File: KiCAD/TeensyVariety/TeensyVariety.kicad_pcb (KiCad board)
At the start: 2 copper layers, 49.5 x 40.5 mm, 36 parts, among them J1 CH1, J2 TRIG INP, J3 LASER, J4 CH2, J5 CH3, J6 CH4 / Decimated Trig, J7 DEBUG, J8 PHOTOTRANSISTOR, Q2 Q_NPN_BCE, U1 Teensy4.0

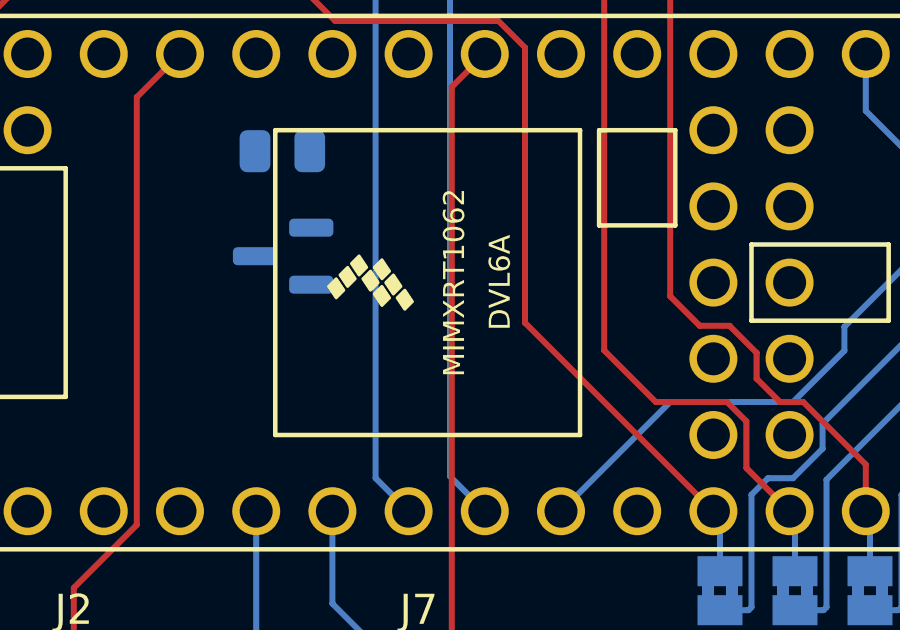
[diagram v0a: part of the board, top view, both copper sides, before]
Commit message: Updated UI and also minor edits to unfinished PCB
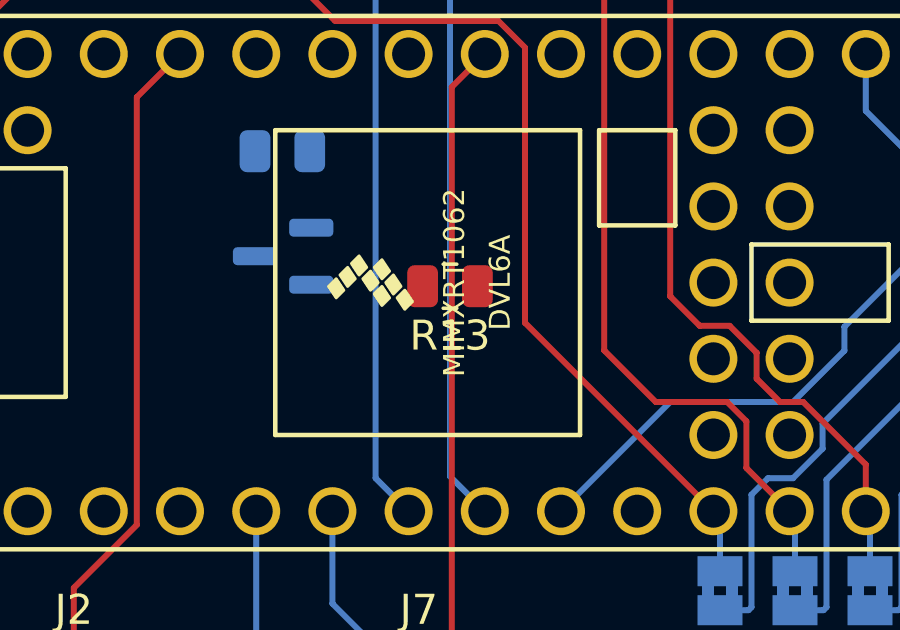
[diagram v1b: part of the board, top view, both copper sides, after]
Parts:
- added R13: 10R, Resistor_SMD:R_0805_2012Metric, F.Cu at (116.0, 70.5)
- R2: value 1K -> 6.7K
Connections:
- Q2 pad 2: /Laser - -> Net-(Q2-C)
